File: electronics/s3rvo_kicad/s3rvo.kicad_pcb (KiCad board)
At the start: 2 copper layers, 69 parts, among them IC1 ADR4540BRZ, IC1 ADR4550BRZ, IC2 AD7685CRMZ, IC3 DRV8703QRHBRQ1, IC4 DRV8703QRHBRQ1, IC4 MP2459GJ-Z, J1 Conn_Enc, J2 Conn_CAN, Q1 CSD18540Q5B, Q2 CSD18540Q5B, Q3 CSD18540Q5B, Q4 CSD18540Q5B, SW1 SW_Push, U1 INA253A2IPWR, U2 STM32F446RCT6, U3 SN65HVD230, U4 XC6206P332MR-G, U8 ADP7142AUJZ-5.0, Y1 X322512MSB4SI

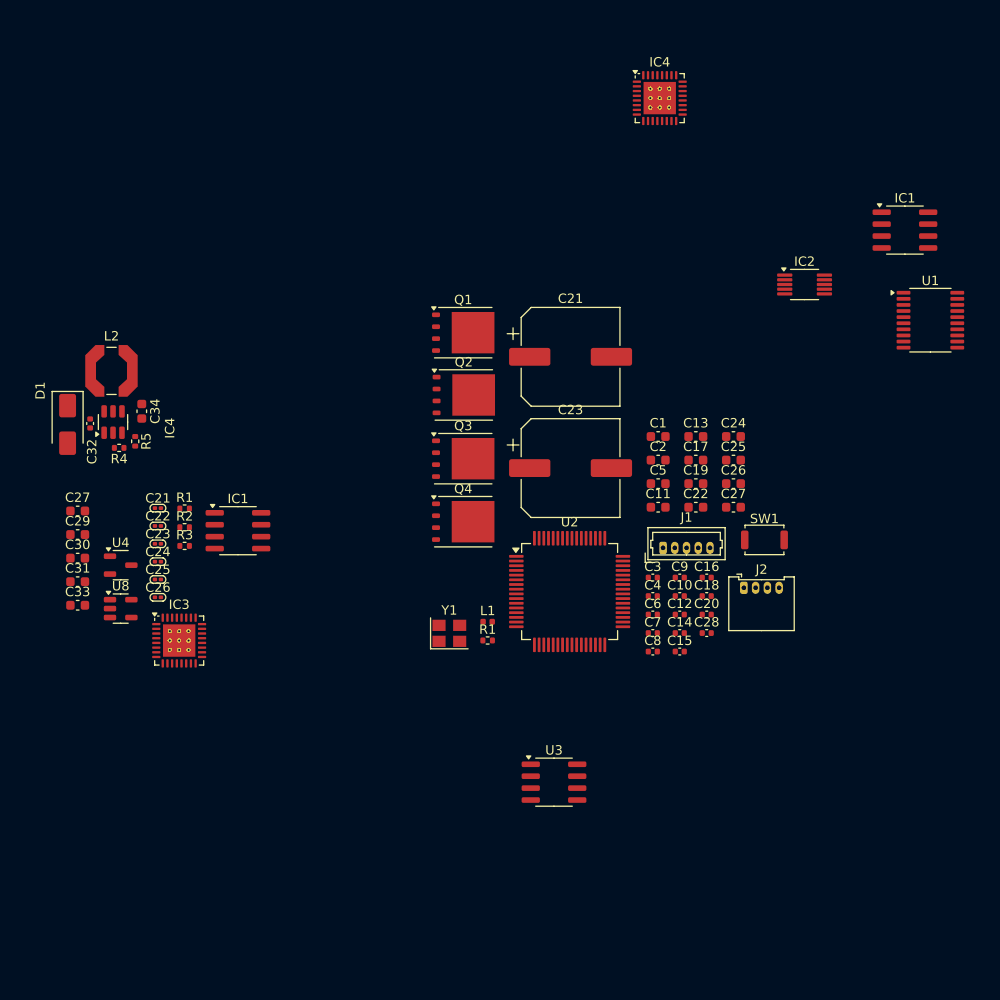
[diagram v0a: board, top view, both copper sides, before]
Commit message: Update
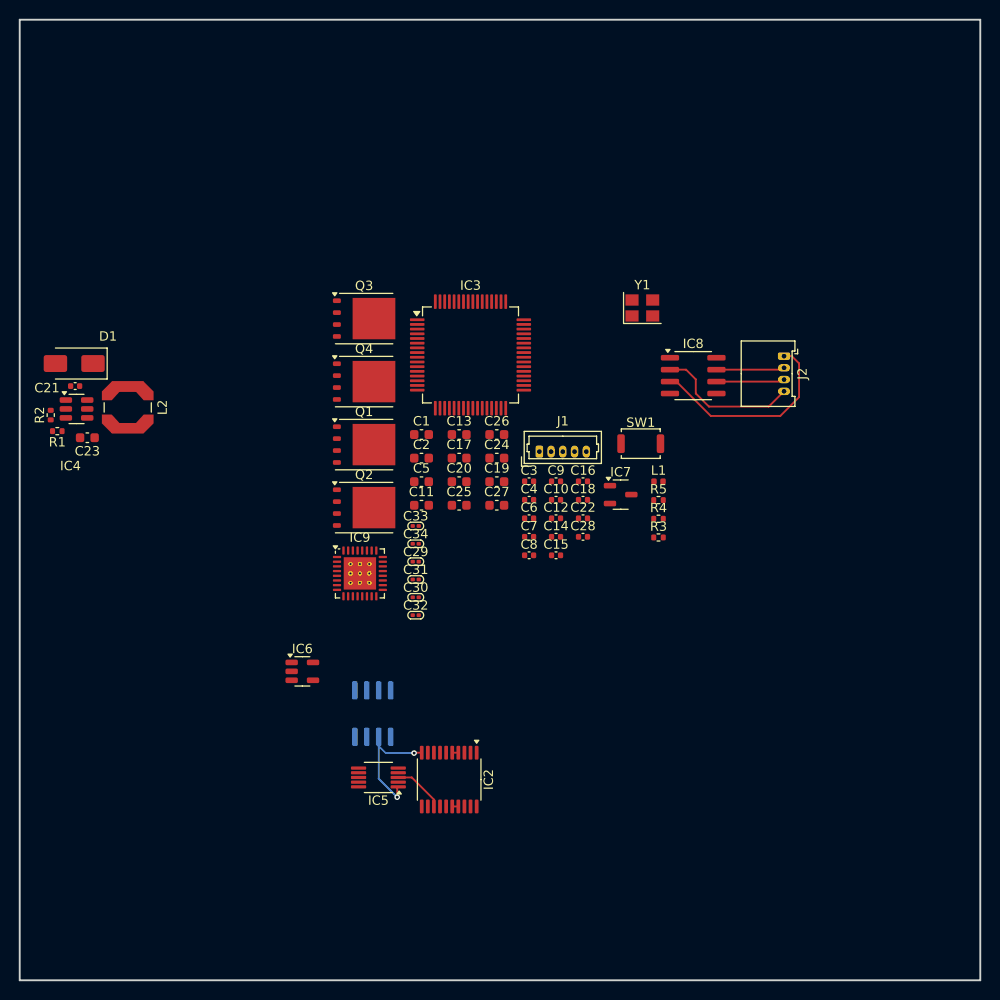
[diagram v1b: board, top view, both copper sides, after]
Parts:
- removed the C21 at (155.4, 73.9)
- removed the C21 at (111.4, 90.0)
- removed the C22 at (168.7, 89.9)
- removed the C22 at (111.4, 91.9)
- removed the C23 at (155.4, 85.8)
- removed the C23 at (111.4, 93.8)
- removed the C24 at (172.7, 82.4)
- removed the C24 at (111.4, 95.7)
- removed the C25 at (172.7, 84.9)
- removed the C25 at (111.4, 97.6)
- removed the C26 at (172.7, 87.4)
- removed the C26 at (111.4, 99.5)
- removed the C27 at (102.9, 90.3)
- removed the C27 at (172.7, 89.9)
- removed the IC1 at (119.9, 92.4)
- removed the IC1 at (191.0, 60.4)
- removed the IC4 at (164.9, 46.4)
- removed the R1 at (114.3, 90.1)
- removed the R1 at (146.5, 104.1)
- removed the R2 at (114.3, 92.0)
- removed U1: INA253A2IPWR, Package_SO:TSSOP-20_4.4x6.5mm_P0.65mm
- removed U2: STM32F446RCT6, Package_QFP:LQFP-64_10x10mm_P0.5mm
- removed U3: SN65HVD230, Package_SO:SOIC-8_3.9x4.9mm_P1.27mm
- removed U4: XC6206P332MR-G, Package_TO_SOT_SMD:SOT-23-3
- removed U8: ADP7142AUJZ-5.0, Package_TO_SOT_SMD:TSOT-23-5
- added C22: 100nF, Capacitor_SMD:C_0402_1005Metric, F.Cu at (156.7, 91.1)
- added C24: 2.2uF, Capacitor_SMD:C_0603_1608Metric, F.Cu at (147.5, 84.7)
- added C25: 1uF, Capacitor_SMD:C_0603_1608Metric, F.Cu at (143.5, 89.7)
- added C26: 1uF, Capacitor_SMD:C_0603_1608Metric, F.Cu at (147.5, 82.2)
- added C27: 2.2uF, Capacitor_SMD:C_0603_1608Metric, F.Cu at (147.5, 89.7)
- added C32: 22uF, PCM_Capacitor_SMD_AKL:C_0201_0603Metric, F.Cu at (138.9, 101.4)
- added C34: 100nF, PCM_Capacitor_SMD_AKL:C_0201_0603Metric, F.Cu at (138.9, 93.8)
- added IC1: ADR4550BRZ, Package_SO:SOIC-8_3.9x4.9mm_P1.27mm, B.Cu at (134.3, 111.9)
- added IC5: AD7685CRMZ, Package_SO:MSOP-10_3x3mm_P0.5mm, F.Cu at (134.9, 118.7)
- added IC6: ADP7142AUJZ-5.0, Package_TO_SOT_SMD:TSOT-23-5, F.Cu at (126.8, 107.4)
- added IC7: XC6206P332MR-G, Package_TO_SOT_SMD:SOT-23-3, F.Cu at (160.7, 88.6)
- added IC8: SN65HVD230, Package_SO:SOIC-8_3.9x4.9mm_P1.27mm, F.Cu at (168.4, 75.9)
- added IC9: DRV8703QRHBRQ1, Package_DFN_QFN:QFN-32-1EP_5x5mm_P0.5mm_EP3.45x3.45mm_ThermalVias, F.Cu at (132.9, 97.0)
- added R4: 10k, Resistor_SMD:R_0402_1005Metric, F.Cu at (164.7, 91.2)
- added R5: 10k, Resistor_SMD:R_0402_1005Metric, F.Cu at (164.7, 89.2)
- C19: value 22uF -> 4.7uF
- C20: value 100nF -> 22uF; footprint Capacitor_SMD:C_0402_1005Metric -> Capacitor_SMD:C_0603_1608Metric
- C29: footprint Capacitor_SMD:C_0603_1608Metric -> PCM_Capacitor_SMD_AKL:C_0201_0603Metric
- C30: value 2.2uF -> 100nF; footprint Capacitor_SMD:C_0603_1608Metric -> PCM_Capacitor_SMD_AKL:C_0201_0603Metric
- C31: value 4.7uF -> 1uF; footprint Capacitor_SMD:C_0603_1608Metric -> PCM_Capacitor_SMD_AKL:C_0201_0603Metric
- C33: value 2.2uF -> 1uF; footprint Capacitor_SMD:C_0603_1608Metric -> PCM_Capacitor_SMD_AKL:C_0201_0603Metric
- IC2: value AD7685CRMZ -> INA253A2IPWR; footprint Package_SO:MSOP-10_3x3mm_P0.5mm -> Package_SO:TSSOP-20_4.4x6.5mm_P0.65mm
- IC3: value DRV8703QRHBRQ1 -> STM32F446RCT6; footprint Package_DFN_QFN:QFN-32-1EP_5x5mm_P0.5mm_EP3.45x3.45mm_ThermalVias -> Package_QFP:LQFP-64_10x10mm_P0.5mm
- moved IC2 64.9 mm to (142.4, 118.9), turned to -90 degrees
- moved R3 50.5 mm to (164.7, 93.1)
- moved IC3 43.5 mm to (144.7, 73.7)
- moved Y1 40.3 mm to (163.0, 68.7)
- moved C33 37.0 mm to (138.9, 91.9)
- moved C30 36.2 mm to (138.9, 99.5)
- moved C29 36.1 mm to (138.9, 95.7)
- moved C31 36.0 mm to (138.9, 97.6)
- moved C20 29.9 mm to (143.5, 87.2)
- moved C13 25.2 mm to (143.5, 82.2)
- moved C17 25.2 mm to (143.5, 84.7)
- moved C1 25.2 mm to (139.5, 82.2)
- moved C11 25.2 mm to (139.5, 89.7)
- moved C2 25.2 mm to (139.5, 84.7)
- moved C5 25.2 mm to (139.5, 87.2)
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- renumbered C32 to C21, C34 to C23, R5 to R1, R4 to R2
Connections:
- C13 pad 1: Net-(IC1-OUT) -> /V_REF
- C15 pad 1: Net-(IC1-OUT) -> /V_REF
- C17 pad 1: Net-(U2-VCAP_1) -> Net-(IC3-VCAP_1)
- C19 pad 1: /V_REF -> VM
- C20 pad 1: +3V3 -> /V_REF
- C29 pad 1: +3V3 -> Net-(IC9-DVDD)
- C30 pad 1: +5V5 -> VM
- C31 pad 1: VM -> /AVDD
- C33 pad 1: +5V -> VM
- C33 pad 2: GND -> Net-(IC9-VCP)
- IC2 pad 1: /V_REF -> /CS_M
- IC2 pad 10: +3V3 -> /V_REF
- IC2 pad 2: +5V -> unconnected-(IC2-IS_N-Pad2)
- IC2 pad 3: /V_CS -> unconnected-(IC2-IS_N-Pad3)
- IC2 pad 4: GND -> Net-(IC2-IN-)
- IC2 pad 5: GND -> Net-(IC2-IN-)
- IC2 pad 6: /SPI_CS -> GND
- IC2 pad 7: /SPI1_MISO -> unconnected-(IC2-DNC1-Pad7)
- IC2 pad 8: /SPI1_SCK -> unconnected-(IC2-NC-Pad8)
- IC2 pad 9: /SPI1_MOSI -> +5V
- IC3 pad 1: GND -> +3V3
- IC3 pad 10: /nFAULT -> unconnected-(IC3-PC2-Pad10)
- IC3 pad 11: /MODE -> unconnected-(IC3-PC3-Pad11)
- IC3 pad 12: Net-(IC3-DVDD) -> unconnected-(IC3-VSSA-Pad12)
- IC3 pad 13: GND -> +3.3VA
- IC3 pad 14: /AVDD -> /ECN_A
- IC3 pad 15: /AVDD -> /ECN_B
- IC3 pad 17: GND -> unconnected-(IC3-PA3-Pad17)
- IC3 pad 18: Net-(IC3-GH1) -> GND
- IC3 pad 19: Net-(IC3-SH1) -> +3V3
- IC3 pad 2: /IN1 -> unconnected-(IC3-PC13-Pad2)
- IC3 pad 20: Net-(IC3-GL1) -> unconnected-(IC3-PA4-Pad20)
- IC3 pad 21: GND -> /SPI1_SCK
- IC3 pad 22: GND -> /SPI1_MISO
- IC3 pad 23: GND -> /SPI1_MOSI
- IC3 pad 24: Net-(IC3-GL2) -> unconnected-(IC3-PC4-Pad24)
- IC3 pad 25: Net-(IC3-SH2) -> unconnected-(IC3-PC5-Pad25)
- IC3 pad 26: Net-(IC3-GH2) -> unconnected-(IC3-PB0-Pad26)
- IC3 pad 27: VM -> unconnected-(IC3-PB1-Pad27)
- IC3 pad 28: VM -> unconnected-(IC3-PB2-Pad28)
- IC3 pad 29: Net-(IC3-VCP) -> unconnected-(IC3-PB10-Pad29)
- IC3 pad 3: /IN2 -> unconnected-(IC3-PC14-Pad3)
- IC3 pad 30: Net-(IC3-CPH) -> Net-(IC3-VCAP_1)
- IC3 pad 31: Net-(IC3-CPL) -> GND
- IC3 pad 32: unconnected-(IC3-NC-Pad32) -> +3V3
- IC3 pad 33: (no net) -> unconnected-(IC3-PB12-Pad33)
- IC3 pad 4: /SDO -> unconnected-(IC3-PC15-Pad4)
- IC3 pad 5: /nSCS -> /RCC_OSC_IN
- IC3 pad 6: /SDI -> /RCC_OSC_OUT
- IC3 pad 7: /SCLK -> /NRST
- IC3 pad 8: /nSLEEP -> unconnected-(IC3-PC0-Pad8)
- IC3 pad 9: /nWDFLT -> unconnected-(IC3-PC1-Pad9)
- J2 pad 1: +5V -> +3V3
- Q1 pad 1: Net-(IC3-SH1) -> /CS_M
- Q1 pad 2: Net-(IC3-SH1) -> /CS_M
- Q1 pad 3: Net-(IC3-SH1) -> /CS_M
- Q1 pad 4: Net-(IC3-GH1) -> Net-(IC9-GH2)
- Q2 pad 4: Net-(IC3-GL1) -> Net-(IC9-GL2)
- Q2 pad 5: Net-(IC3-SH1) -> /CS_M
- Q3 pad 1: Net-(IC3-SH2) -> /CS_P
- Q3 pad 2: Net-(IC3-SH2) -> /CS_P
- Q3 pad 3: Net-(IC3-SH2) -> /CS_P
- Q3 pad 4: Net-(IC3-GH2) -> Net-(IC9-GH1)
- Q4 pad 4: Net-(IC3-GL2) -> Net-(IC9-GL1)
- Q4 pad 5: Net-(IC3-SH2) -> /CS_P
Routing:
- net +3V3: track 0.00 -> 21.6 mm
- net GND: track 0.00 -> 15.3 mm
- net /V_REF: track 0.00 -> 14.3 mm, vias 0 -> 2
- net /CAN_L: track 0.00 -> 7.29 mm
- net /CAN_H: track 0.00 -> 7.28 mm
- net /V_CS: track 0.00 -> 5.51 mm
- net Net-(IC2-IN-): track 0.00 -> 0.65 mm
- net Net-(IC2-IN+): track 0.00 -> 0.65 mm
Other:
- board outline added: 102.3 x 102.3 mm
- copper layers 2 -> 4
